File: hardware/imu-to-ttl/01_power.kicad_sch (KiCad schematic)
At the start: 20 parts, among them J1 BATT IN 2.54 2P, Q1 AO4407C, U4 HT7533-1

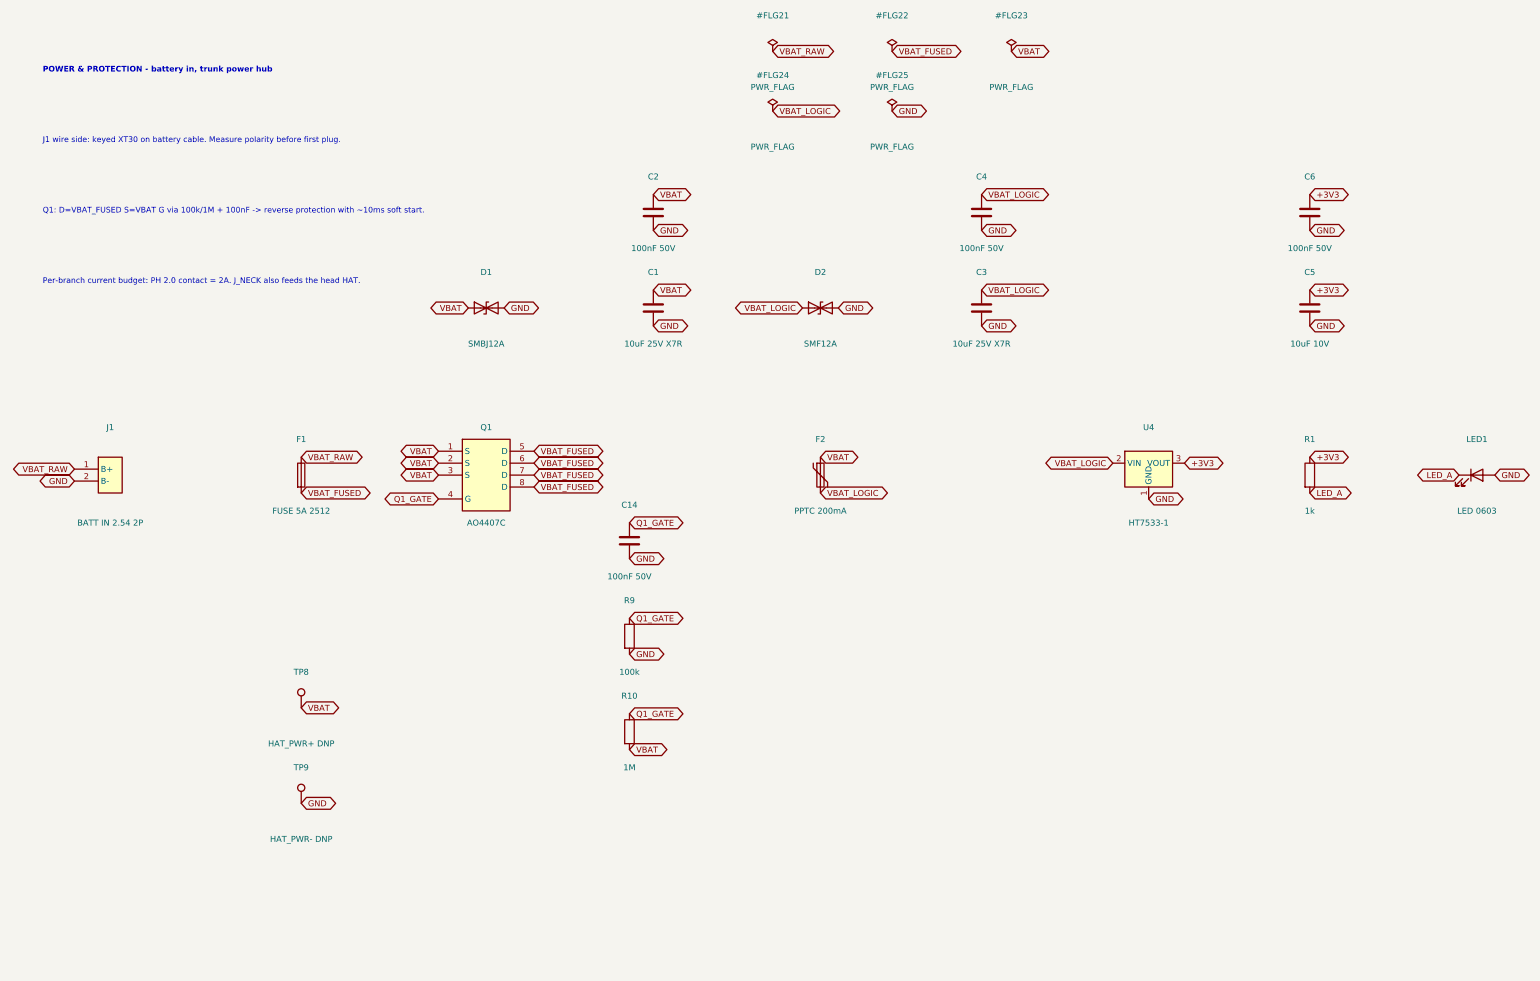
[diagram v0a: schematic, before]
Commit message: sync: 2026-10-12 日常更新
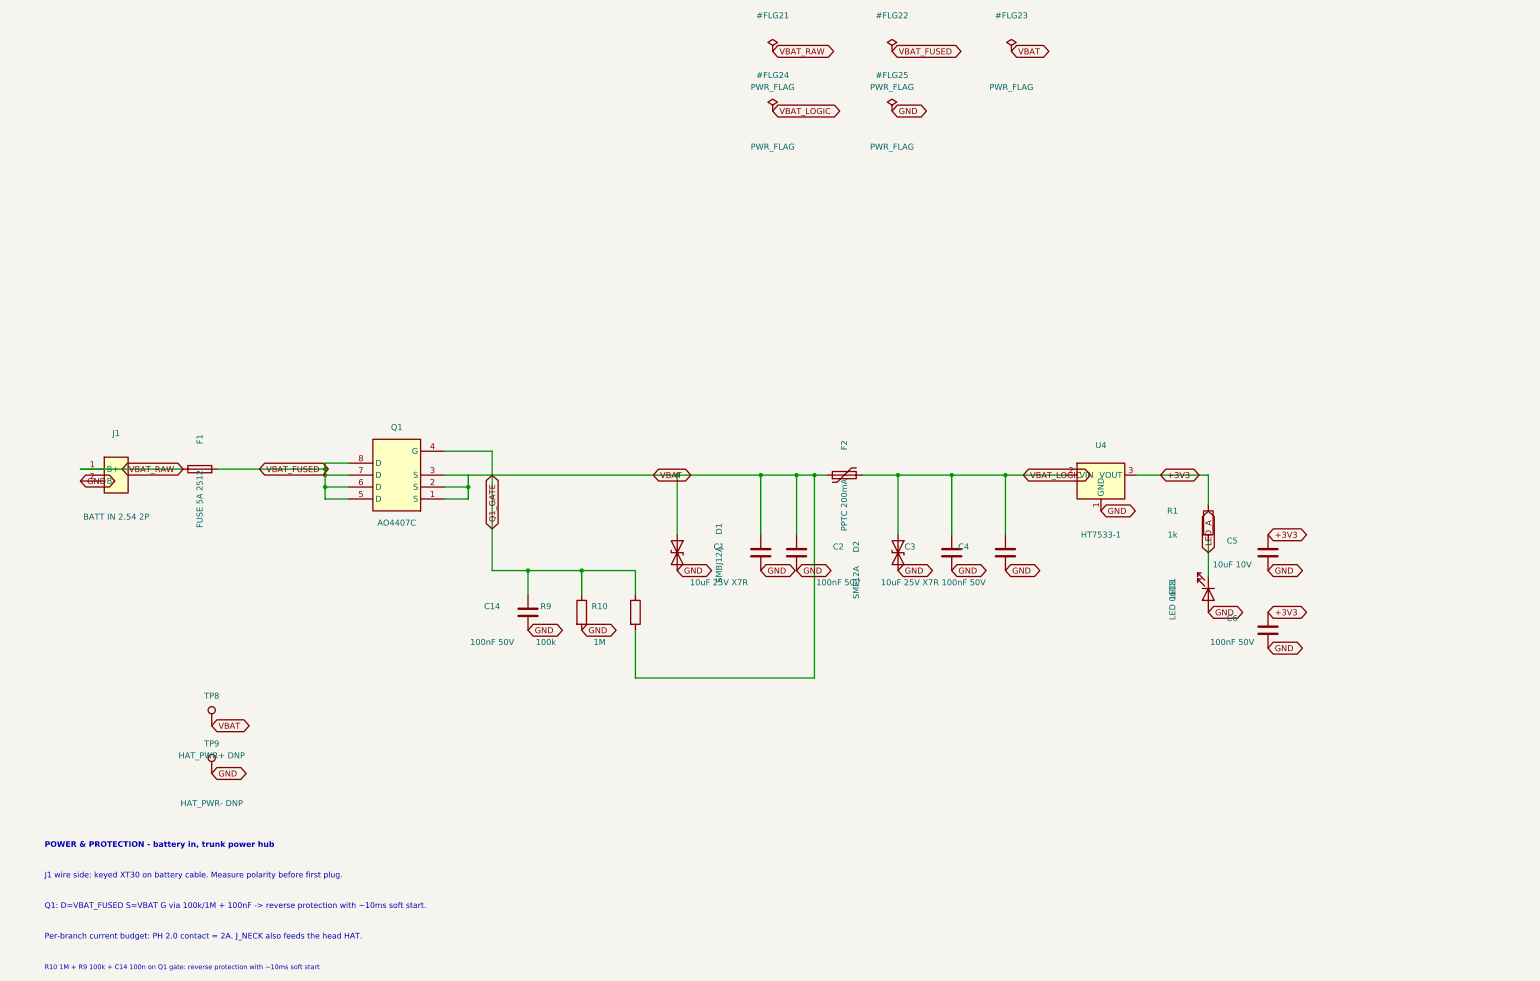
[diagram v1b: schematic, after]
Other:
- note added: "R10 1M + R9 100k + C14 100n on Q1 gate: reverse protection with ~10ms soft start"

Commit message: sync: 2026-10-14 日常更新
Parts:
- J1: footprint TerminalBlock:TerminalBlock_Xinya_XY308-2.54-2P_1x02_P2.54mm_Horizontal -> imu_to_ttl:BattPad_1x02_P3.60mm_Drill1.2mm
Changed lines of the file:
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@@
 	)
 	)
-		(property "Footprint" "TerminalBlock:TerminalBlock_Xinya_XY308-2.54-2P_1x02_P2.54mm_Horizontal"
+		(property "Footprint" "imu_to_ttl:BattPad_1x02_P3.60mm_Drill1.2mm"
 		(at 39.37 110.49 0)
 		(effects

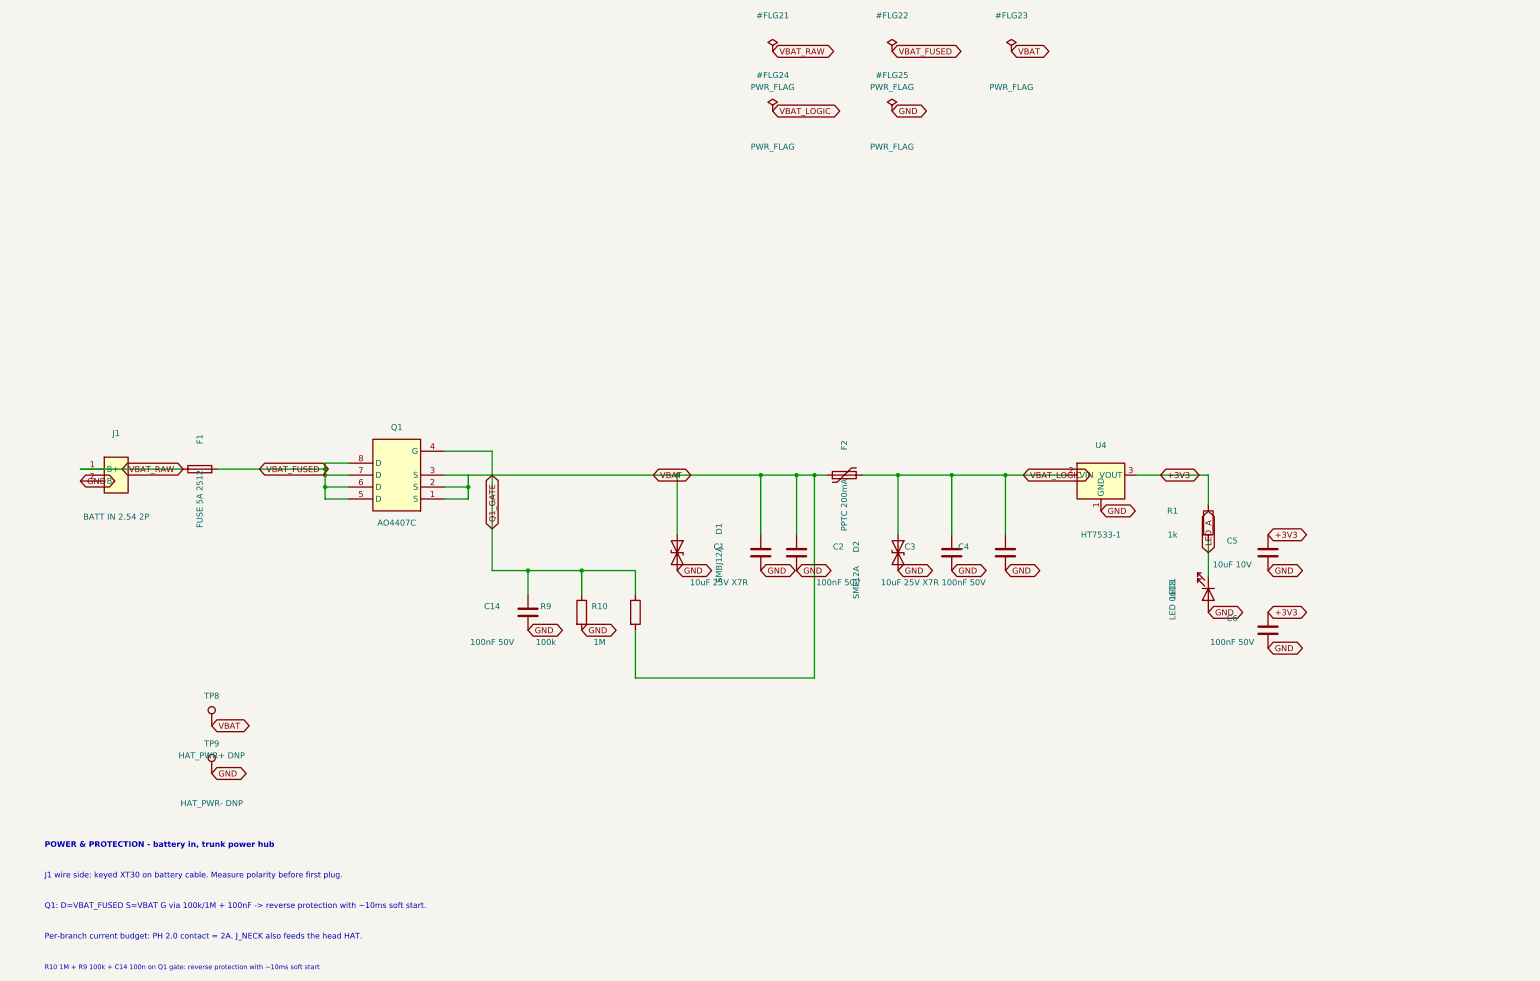
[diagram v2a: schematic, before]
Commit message: sync: 2026-10-15 日常更新
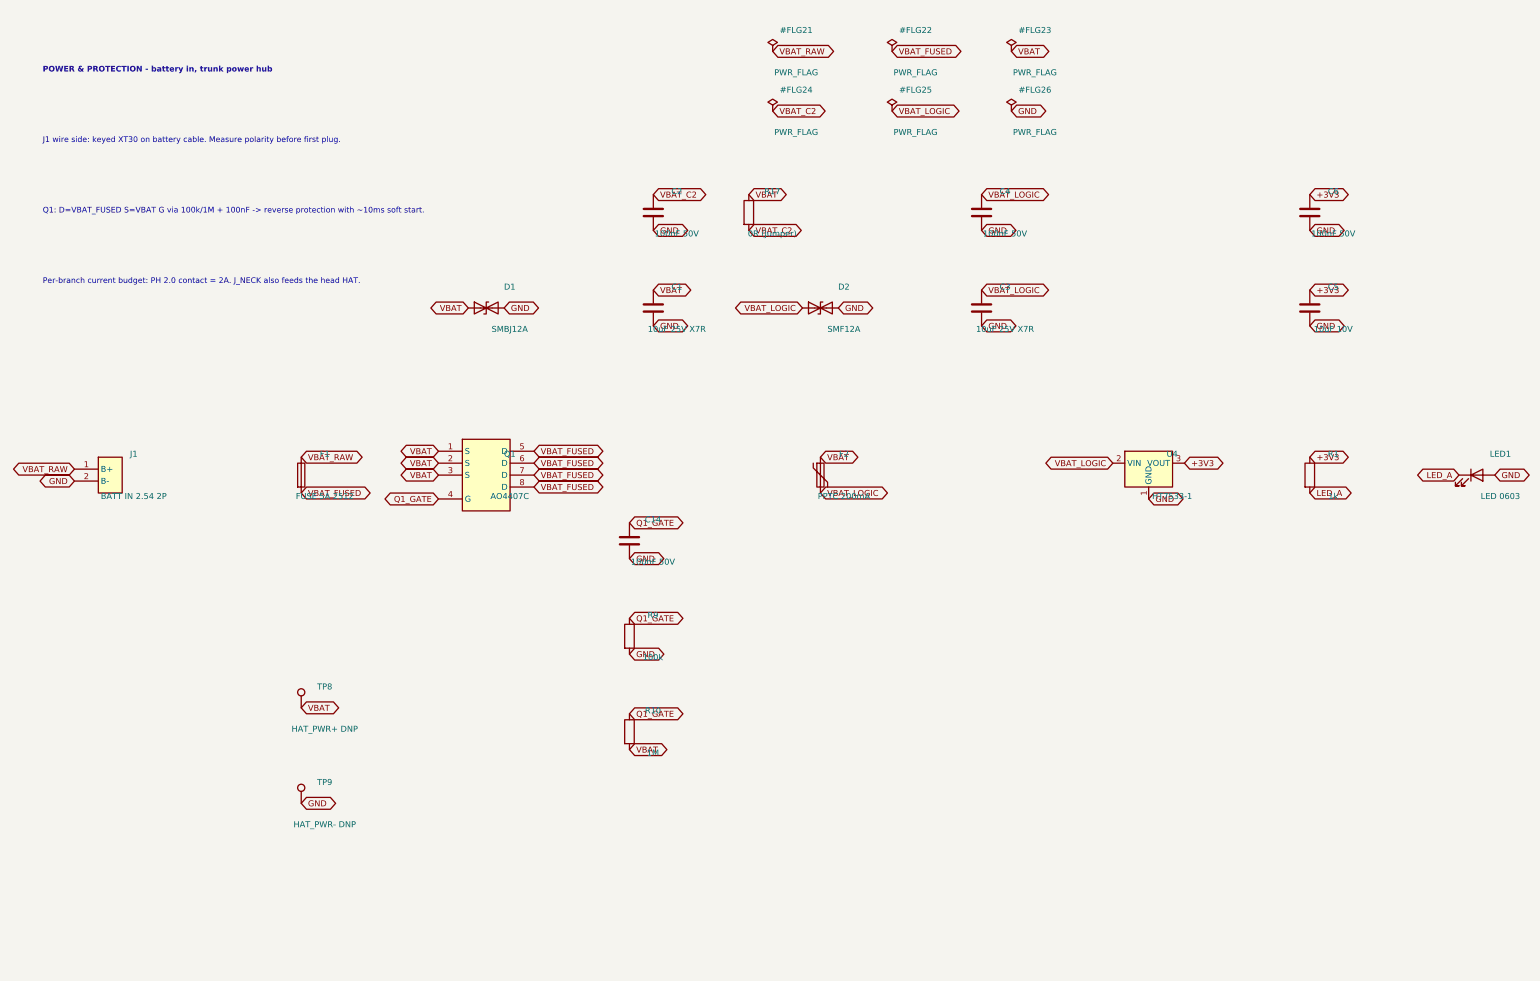
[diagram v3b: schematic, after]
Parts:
- added R17: 0R (jumper), Resistor_SMD:R_0603_1608Metric, symbol Device:R
- J1: footprint imu_to_ttl:BattPad_1x02_P3.60mm_Drill1.2mm -> TerminalBlock:TerminalBlock_Xinya_XY308-2.54-2P_1x02_P2.54mm_Horizontal
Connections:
- net VBAT: now also R17.1; no longer C2.1
- new net VBAT_C2: C2.1, R17.2
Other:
- note removed: "R10 1M + R9 100k + C14 100n on Q1 gate: reverse protection with ~10ms soft start"

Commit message: sync: 2026-10-15 日常更新
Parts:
- J1: footprint TerminalBlock:TerminalBlock_Xinya_XY308-2.54-2P_1x02_P2.54mm_Horizontal -> imu_to_ttl:BattPad_1x02_P3.60mm_Drill1.2mm
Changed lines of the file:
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@@
 	)
 	)
-		(property "Footprint" "TerminalBlock:TerminalBlock_Xinya_XY308-2.54-2P_1x02_P2.54mm_Horizontal"
+		(property "Footprint" "imu_to_ttl:BattPad_1x02_P3.60mm_Drill1.2mm"
 		(at 39.37 110.49 0)
 		(effects

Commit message: sync: 2026-10-15 日常更新
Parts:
- R17: LCSC (none) -> C21189; MPN (none) -> 0603WAF0000T5E
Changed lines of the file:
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@@
 		)
 	)
-	)
+	)		(property "MPN" "0603WAF0000T5E"
+			(at 180.26 50.11 0)
+			(effects
+				(font
+					(size 1.27 1.27)
+				)
+				(hide yes)
+			)
+		)
+		(property "LCSC" "C21189"
+			(at 180.26 50.11 0)
+			(effects
+				(font
+					(size 1.27 1.27)
+				)
+				(hide yes)
+			)
+		)
 		(property "Footprint" "Resistor_SMD:R_0603_1608Metric"
 		(at 175.26 54.61 0)

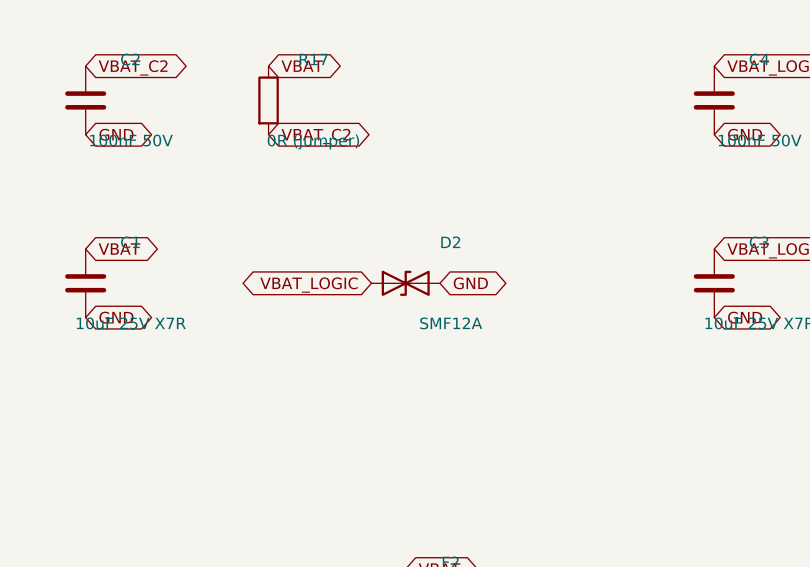
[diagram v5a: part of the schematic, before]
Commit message: sync: 2026-10-21 日常更新
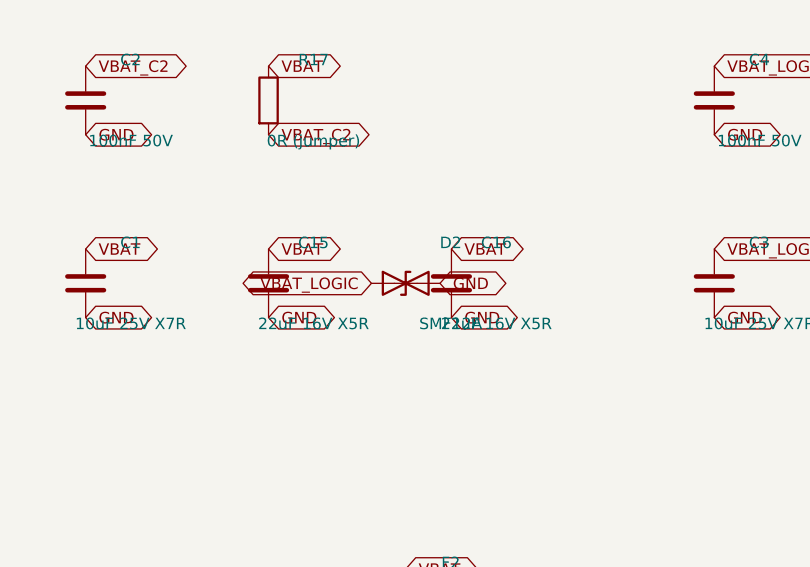
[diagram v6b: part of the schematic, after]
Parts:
- added C15, C16: 22uF 16V X5R, Capacitor_SMD:C_1210_3225Metric, symbol Device:C
- J1: LCSC C474920 -> (none); MPN KF128-2.54-2P -> (none)
- R17: LCSC C21189 -> (none); MPN 0603WAF0000T5E -> (none)
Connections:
- net GND: now also C15.2, C16.2
- net VBAT: now also C15.1, C16.1
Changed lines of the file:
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@@
+	)
+	)
+	(global_label "VBAT"
+		(shape bidirectional)
+		(at 175.26 71.12 0)
+		(fields_autoplaced yes)
+		(effects
+		(font
+			(size 1.27 1.27)
+		)
+			(justify left)
+	)
+	)
+	(global_label "GND"
+		(shape bidirectional)
+		(at 175.26 78.74 0)
+		(fields_autoplaced yes)
+		(effects
+		(font
+			(size 1.27 1.27)
+		)
+			(justify left)
+	)
+	)
+	(global_label "VBAT"
+		(shape bidirectional)
+		(at 195.58 71.12 0)
+		(fields_autoplaced yes)
+		(effects
+		(font
+			(size 1.27 1.27)
+		)
+			(justify left)
+	)
+	)
+	(global_label "GND"
+		(shape bidirectional)
+		(at 195.58 78.74 0)
+		(fields_autoplaced yes)
+		(effects
+		(font
+			(size 1.27 1.27)
+		)
+			(justify left)
 	)
 	)
@@
 	)
 	)
-		(property "MPN" "KF128-2.54-2P"
-		(at 39.37 110.49 0)
-		(effects
-		(font
-			(size 1.27 1.27)
-		)
-			(hide yes)
-	)
-	)
-		(property "LCSC" "C474920"
-		(at 39.37 110.49 0)
-		(effects
-		(font
-			(size 1.27 1.27)
-		)
-			(hide yes)
-	)
-	)
 		(pin "1"
 		)
@@
 	(symbol
 		(lib_id "Device:C")
+		(at 175.26 74.93 0)
+		(unit 1)
+		(exclude_from_sim no)
+		(in_bom yes)
+		(on_board yes)
+		(dnp no)
+		(property "Reference" "C15"
+		(at 180.26 70.43 0)
+		(effects
+		(font
+			(size 1.27 1.27)
+		)
+	)
+	)
+		(property "Value" "22uF 16V X5R"
+		(at 180.26 79.43 0)
+		(effects
+		(font
+			(size 1.27 1.27)
+		)
+	)
+	)
+		(property "Footprint" "Capacitor_SMD:C_1210_3225Metric"
+		(at 175.26 74.93 0)
+		(effects
+		(font
+			(size 1.27 1.27)
+		)
+			(hide yes)
+	)
+	)
+		(property "Datasheet" "~"
+		(at 175.26 74.93 0)
+		(effects
+		(font
+			(size 1.27 1.27)
+		)
+			(hide yes)
+	)
+	)
+		(property "Description" "v3.7 servo surge bulk (dxl_hub 1000uF 的贴片化替代)"
+		(at 175.26 74.93 0)
+		(effects
+		(font
+			(size 1.27 1.27)
+		)
+			(hide yes)
+	)
+	)
+		(property "MPN" "EMK325BJ226KMHP"
+		(at 175.26 74.93 0)
+		(effects
+		(font
+			(size 1.27 1.27)
+		)
+			(hide yes)
+	)
+	)
+		(property "LCSC" "C359910"
+		(at 175.26 74.93 0)
+		(effects
+		(font
+			(size 1.27 1.27)
+		)
+			(hide yes)
+	)
+	)
+		(pin "1"
+		)
+		(pin "2"
+		)
+		(instances
+			(project "imu_to_ttl"
+				(path "/3d3ee743-797d-5481-a518-f87a3584d0e2/b90fe5c0-5dba-508d-a7d0-e14a681a083e/5d4efe53-e5ce-5b26-b125-f6a670b3ba8e"
+					(reference "C15")
+					(unit 1)
+				)
+			)
+		)
+	)
+	(symbol
+		(lib_id "Device:C")
+		(at 195.58 74.93 0)
+		(unit 1)
+		(exclude_from_sim no)
+		(in_bom yes)
+		(on_board yes)
+		(dnp no)
+		(property "Reference" "C16"
+		(at 200.58 70.43 0)
+		(effects
+		(font
+			(size 1.27 1.27)
+		)
+	)
+	)
+		(property "Value" "22uF 16V X5R"
+		(at 200.58 79.43 0)
+		(effects
+		(font
+			(size 1.27 1.27)
+		)
+	)
+	)
+		(property "Footprint" "Capacitor_SMD:C_1210_3225Metric"
+		(at 195.58 74.93 0)
+		(effects
+		(font
+			(size 1.27 1.27)
+		)
+			(hide yes)
+	)
+	)
+		(property "Datasheet" "~"
+		(at 195.58 74.93 0)
+		(effects
+		(font
+			(size 1.27 1.27)
+		)
+			(hide yes)
+	)
+	)
+		(property "Description" ""
+		(at 195.58 74.93 0)
+		(effects
+		(font
+			(size 1.27 1.27)
+		)
+			(hide yes)
+	)
+	)
+		(property "MPN" "EMK325BJ226KMHP"
+		(at 195.58 74.93 0)
+		(effects
+		(font
+			(size 1.27 1.27)
+		)
+			(hide yes)
+	)
+	)
+		(property "LCSC" "C359910"
+		(at 195.58 74.93 0)
+		(effects
+		(font
+			(size 1.27 1.27)
+		)
+			(hide yes)
+	)
+	)
+		(pin "1"
+		)
+		(pin "2"
+		)
+		(instances
+			(project "imu_to_ttl"
+				(path "/3d3ee743-797d-5481-a518-f87a3584d0e2/b90fe5c0-5dba-508d-a7d0-e14a681a083e/fa732b00-2ebc-5e7b-81f1-ce7643eb12d2"
+					(reference "C16")
+					(unit 1)
+				)
+			)
+		)
+	)
+	(symbol
+		(lib_id "Device:C")
 		(at 154.94 54.61 0)
 		(unit 1)
@@
 		)
 	)
-	)		(property "MPN" "0603WAF0000T5E"
-			(at 180.26 50.11 0)
-			(effects
-				(font
-					(size 1.27 1.27)
-				)
-				(hide yes)
-			)
-		)
-		(property "LCSC" "C21189"
-			(at 180.26 50.11 0)
-			(effects
-				(font
-					(size 1.27 1.27)
-				)
-				(hide yes)
-			)
-		)
+	)
 		(property "Footprint" "Resistor_SMD:R_0603_1608Metric"
 		(at 175.26 54.61 0)
